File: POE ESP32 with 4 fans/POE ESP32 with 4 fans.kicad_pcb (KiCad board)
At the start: 2 copper layers, 137.5 x 89 mm, 15 parts, among them J10 Conn_01x04_Pin, J11 Conn_01x04_Pin, J12 Conn_01x04_Pin, J13 Conn_01x04_Pin, J14 Conn_01x04_Pin, J15 Conn_01x03_Pin, J16 Conn_01x03_Pin, J17 Conn_01x03_Pin, J18 Conn_01x03_Pin, J19 Conn_01x03_Pin, J20 Conn_01x03_Pin, J5 Conn_01x07_Pin, J6 Conn_01x06_Pin, J9 Conn_01x04_Pin, U7 74HCT04

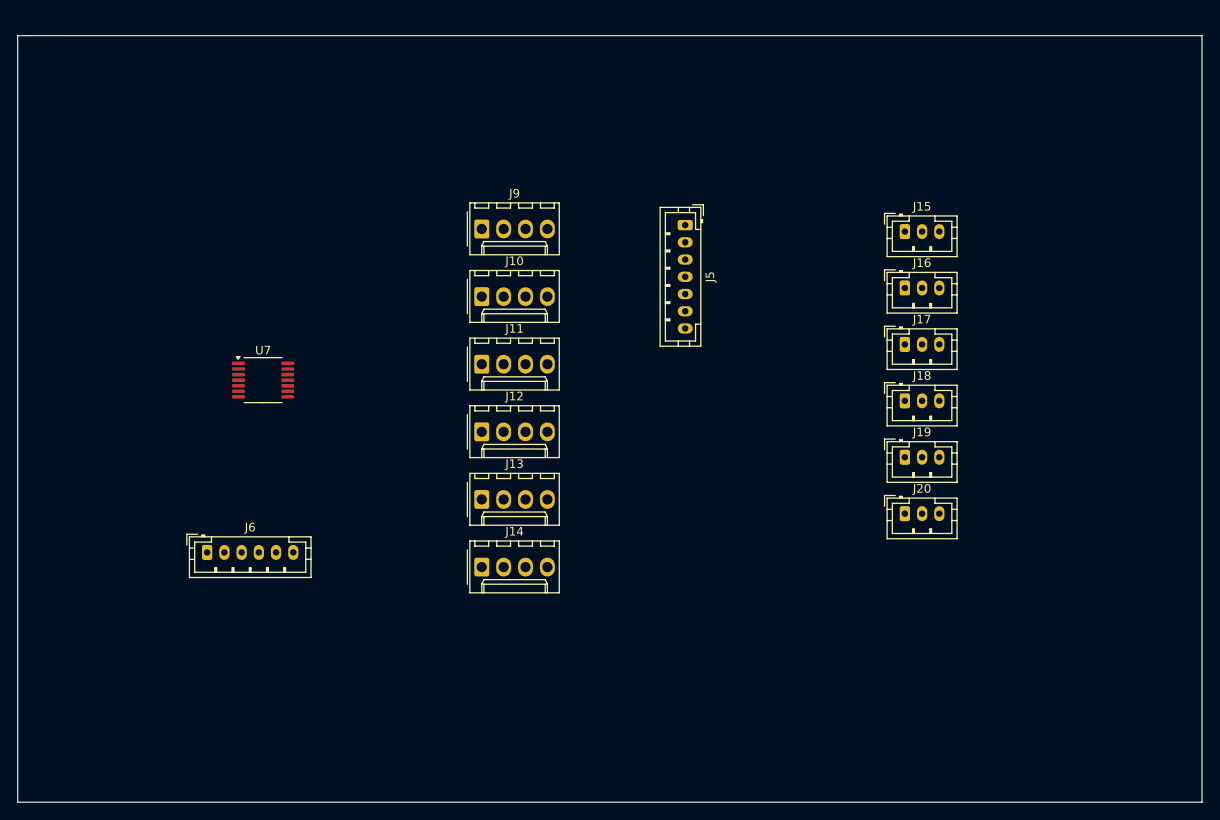
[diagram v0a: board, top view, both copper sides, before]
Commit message: Added PCB
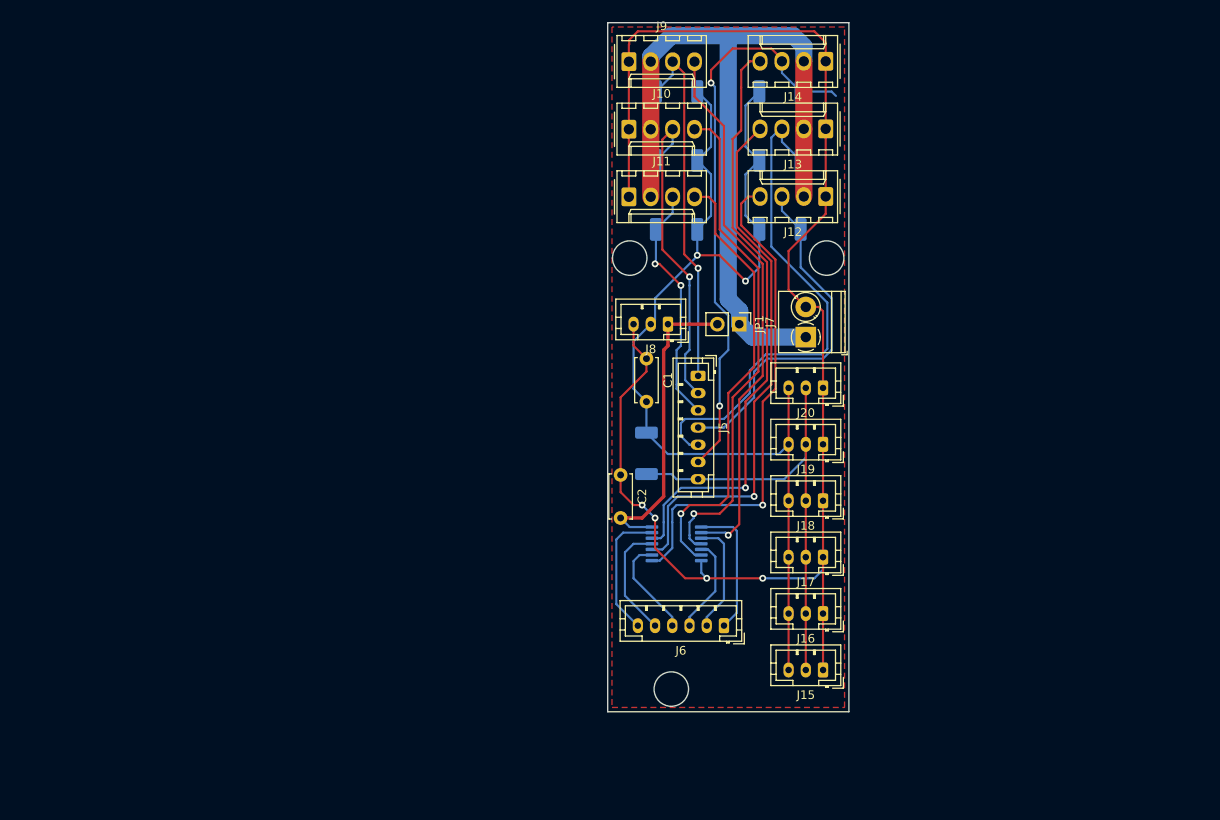
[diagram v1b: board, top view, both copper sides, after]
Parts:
- added C1: 100 nF, Capacitor_THT:C_Disc_D5.0mm_W2.5mm_P5.00mm, F.Cu at (145.5, 83.5)
- added C2: 100 nF, Capacitor_THT:C_Disc_D5.0mm_W2.5mm_P5.00mm, F.Cu at (142.5, 97.0)
- added J7: Conn_01x02_Pin, TerminalBlock_Phoenix:TerminalBlock_Phoenix_PT-1,5-2-3.5-H_1x02_P3.50mm_Horizontal, F.Cu at (164.0, 81.0)
- added J8: Conn_01x03_Pin, Connector_JST:JST_PH_B3B-PH-K_1x03_P2.00mm_Vertical, F.Cu at (148.0, 79.5)
- added JP1: Jumper_2_Open, Connector_PinHeader_2.54mm:PinHeader_1x02_P2.54mm_Vertical, F.Cu at (156.3, 79.5)
- added R1: 10k, Resistor_SMD:R_2010_5025Metric_Pad1.40x2.65mm_HandSolder, B.Cu at (161.0, 52.5)
- added R2: 10k, Resistor_SMD:R_2010_5025Metric_Pad1.40x2.65mm_HandSolder, B.Cu at (161.0, 60.5)
- added R3: 10k, Resistor_SMD:R_2010_5025Metric_Pad1.40x2.65mm_HandSolder, B.Cu at (161.0, 68.5)
- added R4: 10k, Resistor_SMD:R_2010_5025Metric_Pad1.40x2.65mm_HandSolder, B.Cu at (149.0, 68.5)
- added R5: 10k, Resistor_SMD:R_2010_5025Metric_Pad1.40x2.65mm_HandSolder, B.Cu at (149.0, 60.5)
- added R6: 10k, Resistor_SMD:R_2010_5025Metric_Pad1.40x2.65mm_HandSolder, B.Cu at (149.0, 52.5)
- added R7: 4,7k, Resistor_SMD:R_2010_5025Metric_Pad1.40x2.65mm_HandSolder, B.Cu at (145.5, 94.5)
- U7: moved to B.Cu
- moved J14 71.0 mm to (166.3, 49.0), turned to 180 degrees
- moved J6 60.6 mm to (154.5, 114.5), turned to 180 degrees
- moved J13 58.7 mm to (166.3, 56.8), turned to 180 degrees
- moved J15 51.8 mm to (166.0, 119.7), turned to 180 degrees
- moved U7 51.6 mm to (149.0, 105.0), turned to 180 degrees
- moved J12 48.4 mm to (166.3, 64.7), turned to 180 degrees
- moved J16 39.0 mm to (166.0, 113.1), turned to 180 degrees
- moved J17 26.5 mm to (166.0, 106.5), turned to 180 degrees
- moved J11 25.9 mm to (143.5, 64.7)
- moved J10 25.9 mm to (143.5, 56.9)
- moved J9 25.9 mm to (143.5, 49.0)
- moved J5 17.6 mm to (151.5, 85.5)
- moved J20 17.4 mm to (166.0, 86.9), turned to 180 degrees
- moved J18 15.0 mm to (166.0, 100.0), turned to 180 degrees
- moved J19 9.62 mm to (166.0, 93.5), turned to 180 degrees
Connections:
- net Net-(J10-Pin_1) renamed /Signal conditioning/GND
- net Net-(J10-Pin_2) renamed /Signal conditioning/FanSupply
- U7 pad 14: Net-(J8-Pin_1) -> /Signal conditioning/Supply5V
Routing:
- net /Signal conditioning/GND: track 0.00 -> 174.4 mm, vias 0 -> 4
- net Net-(J15-Pin_3): track 0.00 -> 128.8 mm, vias 0 -> 2
- net /Signal conditioning/FanSupply: track 0.00 -> 95.4 mm
- net Net-(J14-Pin_4): track 0.00 -> 69.6 mm, vias 0 -> 1
- net Net-(J14-Pin_3): track 0.00 -> 66.5 mm, vias 0 -> 2
- net Net-(J13-Pin_4): track 0.00 -> 63.2 mm, vias 0 -> 1
- net Net-(J9-Pin_4): track 0.00 -> 63.2 mm, vias 0 -> 1
- net Net-(J13-Pin_3): track 0.00 -> 59.5 mm
- net Net-(J10-Pin_4): track 0.00 -> 58.3 mm, vias 0 -> 1
- net Net-(J12-Pin_4): track 0.00 -> 58.0 mm, vias 0 -> 1
- net Net-(J15-Pin_2): track 0.00 -> 54.1 mm
- net Net-(J11-Pin_4): track 0.00 -> 52.4 mm, vias 0 -> 1
- net Net-(J5-Pin_1): track 0.00 -> 42.0 mm, vias 0 -> 1
- net Net-(J12-Pin_3): track 0.00 -> 41.2 mm
- net Net-(J10-Pin_3): track 0.00 -> 37.7 mm, vias 0 -> 1
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- added copper zone on F.Cu, net /Signal conditioning/GND
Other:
- board size 137.5 x 89 mm -> 28 x 80 mm
